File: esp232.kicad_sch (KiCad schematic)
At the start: 18 parts, among them J1 RS232-Connector, J2 External-PWR, J3 Spare IO, U1 MOUDLE-SEEEDUINO-XIAO-ESP32C3, U2 MAX3232

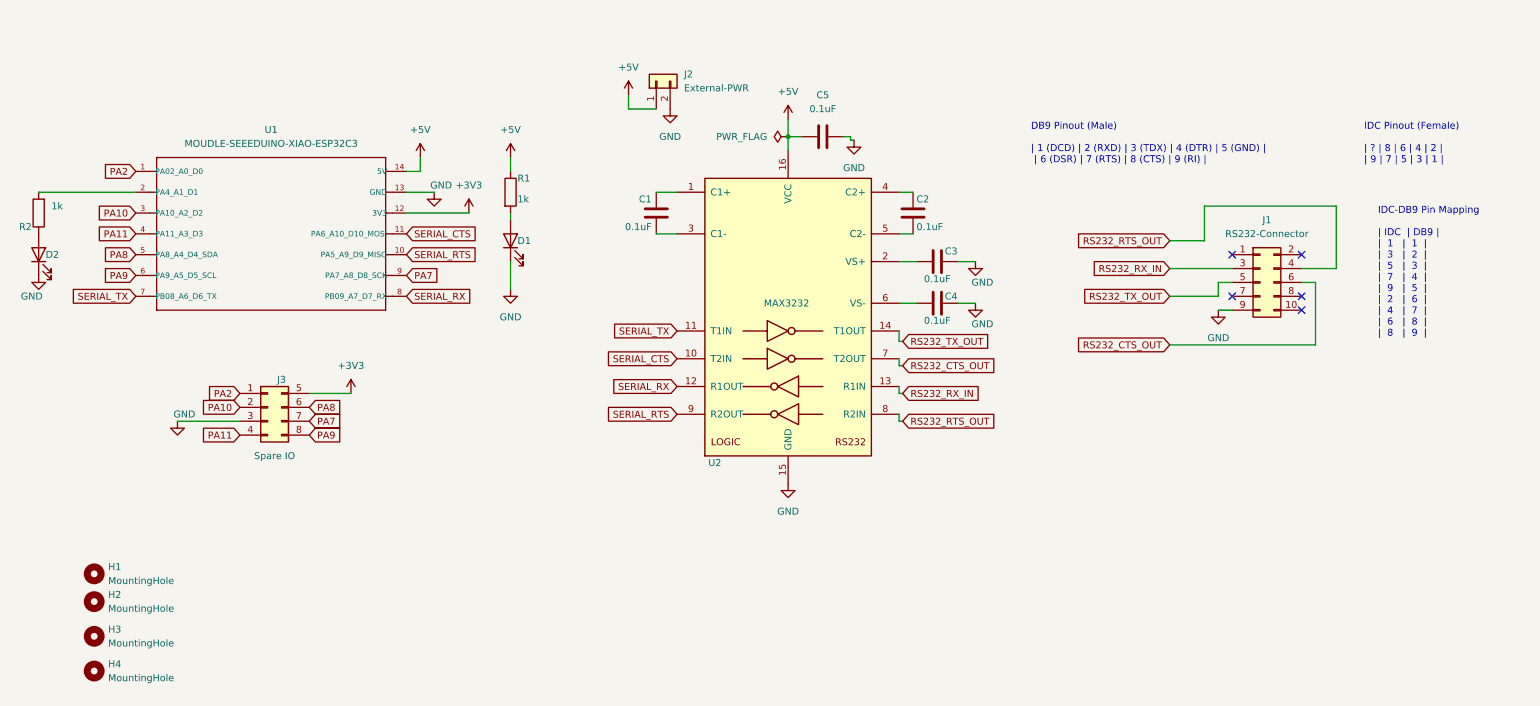
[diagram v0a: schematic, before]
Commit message: small layout improvements
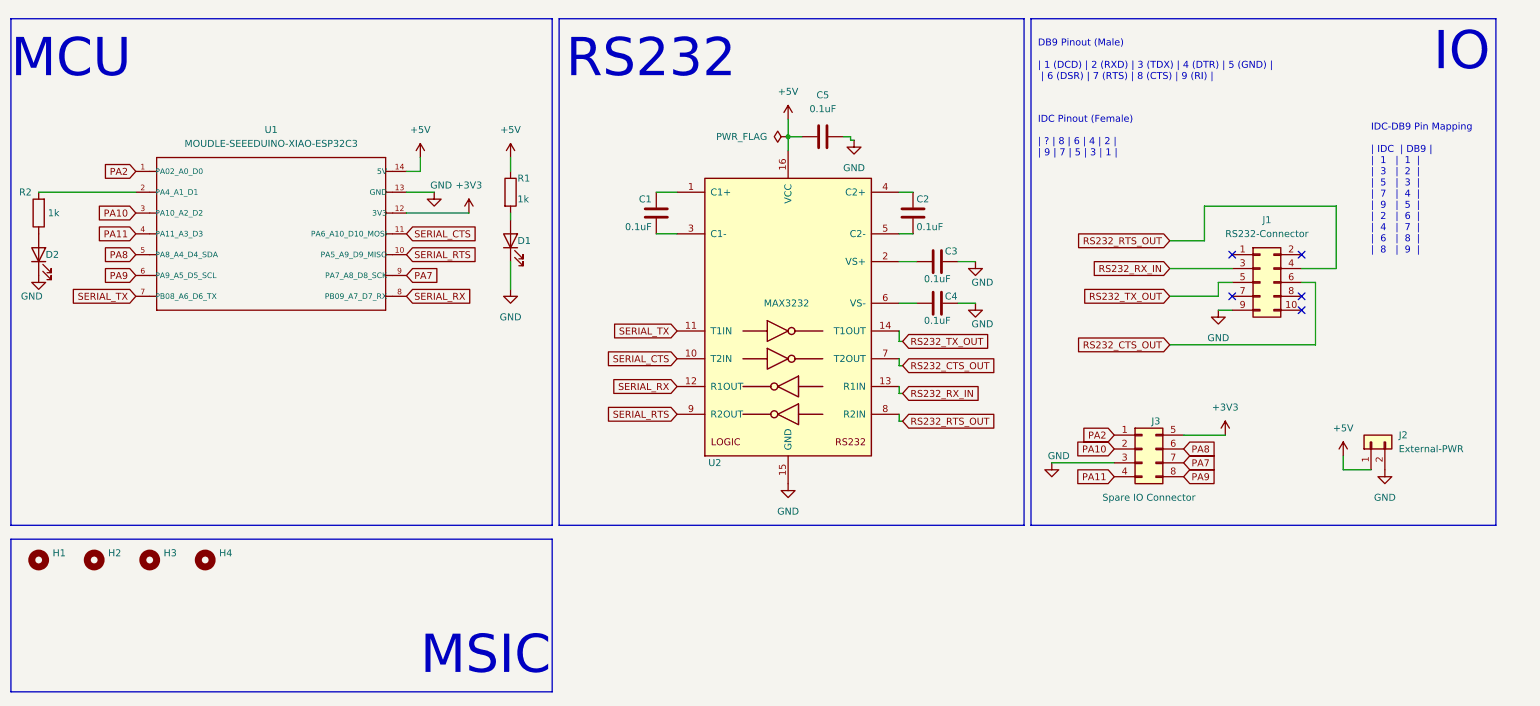
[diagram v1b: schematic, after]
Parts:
- J3: value Spare IO -> Spare IO Connector
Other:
- note added: "IO"
- note added: "MCU"
- note added: "MSIC"
- note added: "RS232"
- moved on the sheet: H1, H2, H3, H4, J2, J3
